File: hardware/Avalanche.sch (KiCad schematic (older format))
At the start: 18 parts

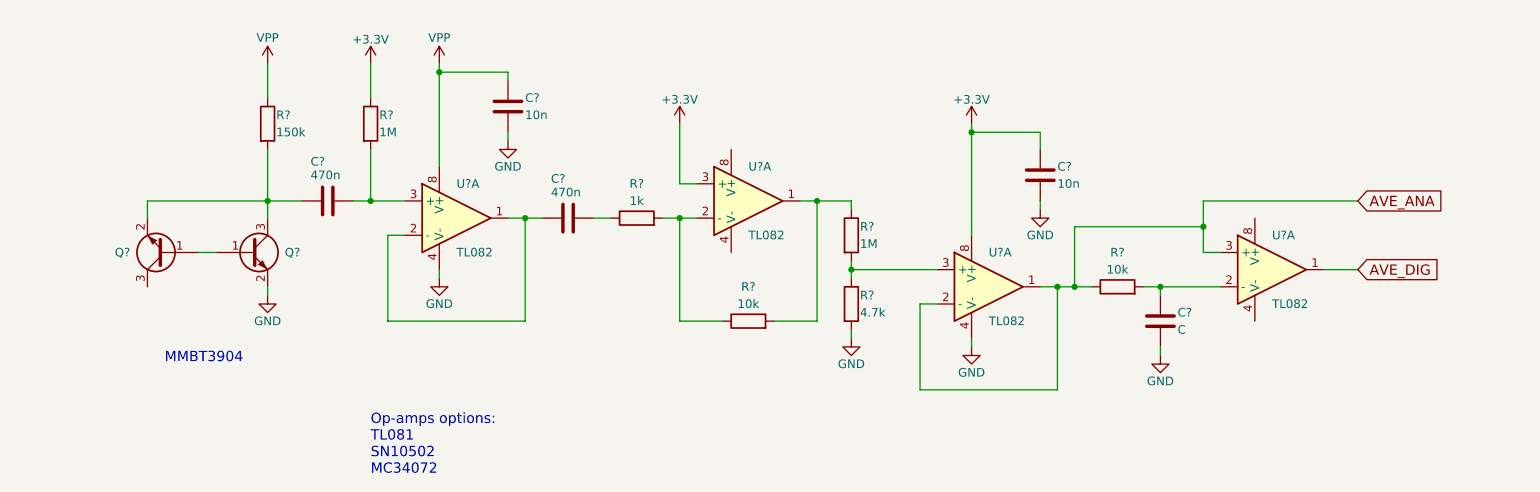
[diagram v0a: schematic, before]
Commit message: IDs, footprints, DRC
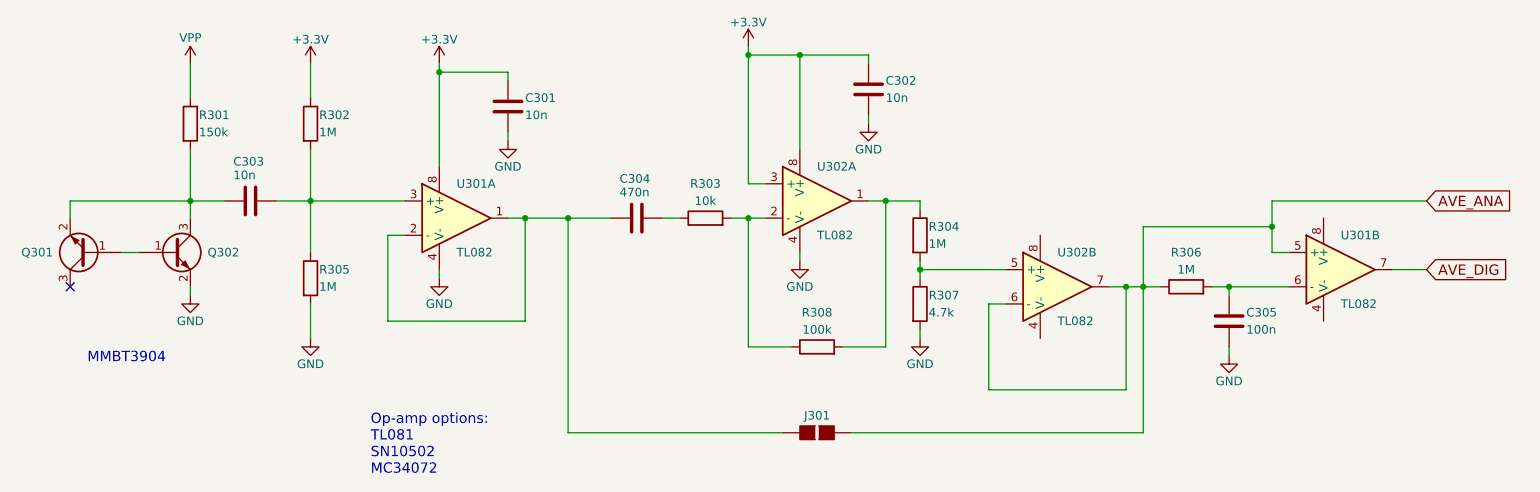
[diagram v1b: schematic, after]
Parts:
- removed U? (x2): TL082, symbol TL082
- added J301: GS2, Connectors:GS2, symbol GS2
- added R305: 1M, Resistors_SMD:R_0603_HandSoldering, symbol R
- added unit 2 of U301
- added unit 2 of U302
- C301, C302, C304: renamed from C?; footprint (none) -> Capacitors_SMD:C_0603_HandSoldering
- C303: renamed from C?; value 470n -> 10n; footprint (none) -> Capacitors_SMD:C_0603_HandSoldering
- C305: renamed from C?; value C -> 100n; footprint (none) -> Capacitors_SMD:C_0603_HandSoldering
- Q301, Q302: renamed from Q?; footprint (none) -> TO_SOT_Packages_SMD:SOT-23
- R301, R302, R304, R307: renamed from R?; footprint (none) -> Resistors_SMD:R_0603_HandSoldering
- R303: renamed from R?; value 1k -> 10k; footprint (none) -> Resistors_SMD:R_0603_HandSoldering
- R306: renamed from R?; value 10k -> 1M; footprint (none) -> Resistors_SMD:R_0603_HandSoldering
- R308: renamed from R?; value 10k -> 100k; footprint (none) -> Resistors_SMD:R_0603_HandSoldering
- U301, U302: renamed from U?; footprint (none) -> Housings_SOIC:SOIC-8_3.9x4.9mm_Pitch1.27mm
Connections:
- net +3V3: now also C301.1, U301.8 (V+), U302.8 (V+)
- net AVE_ANA: now also J301.2 (G2), U301.5 (+), U302.6 (-), U302.7
- net AVE_DIG: now also U301.7
- net GND: now also U302.4 (V-), R305.2
- net VPP: no longer C301.1, U301.8 (V+)
- net at C303.2, R302.2, U301.3 (+): now also R305.1
- net at R304.2, R307.1: now also U302.5 (+)
- net at C304.1, U301.1, U301.2 (-): now also J301.1 (G1)
- net at C305.1, R306.2: now also U301.6 (-)
- no-connect marks 0 -> 1
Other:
- note added: "Op-amp options:\nTL081\nSN10502\nMC34072"
- note removed: "Op-amps options:\nTL081\nSN10502\nMC34072"
- moved on the sheet: C302, C303, C304, C305, Q301, Q302, R301, R302, R303, R304, R306, R307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
